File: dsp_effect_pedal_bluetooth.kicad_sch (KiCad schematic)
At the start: 1 part

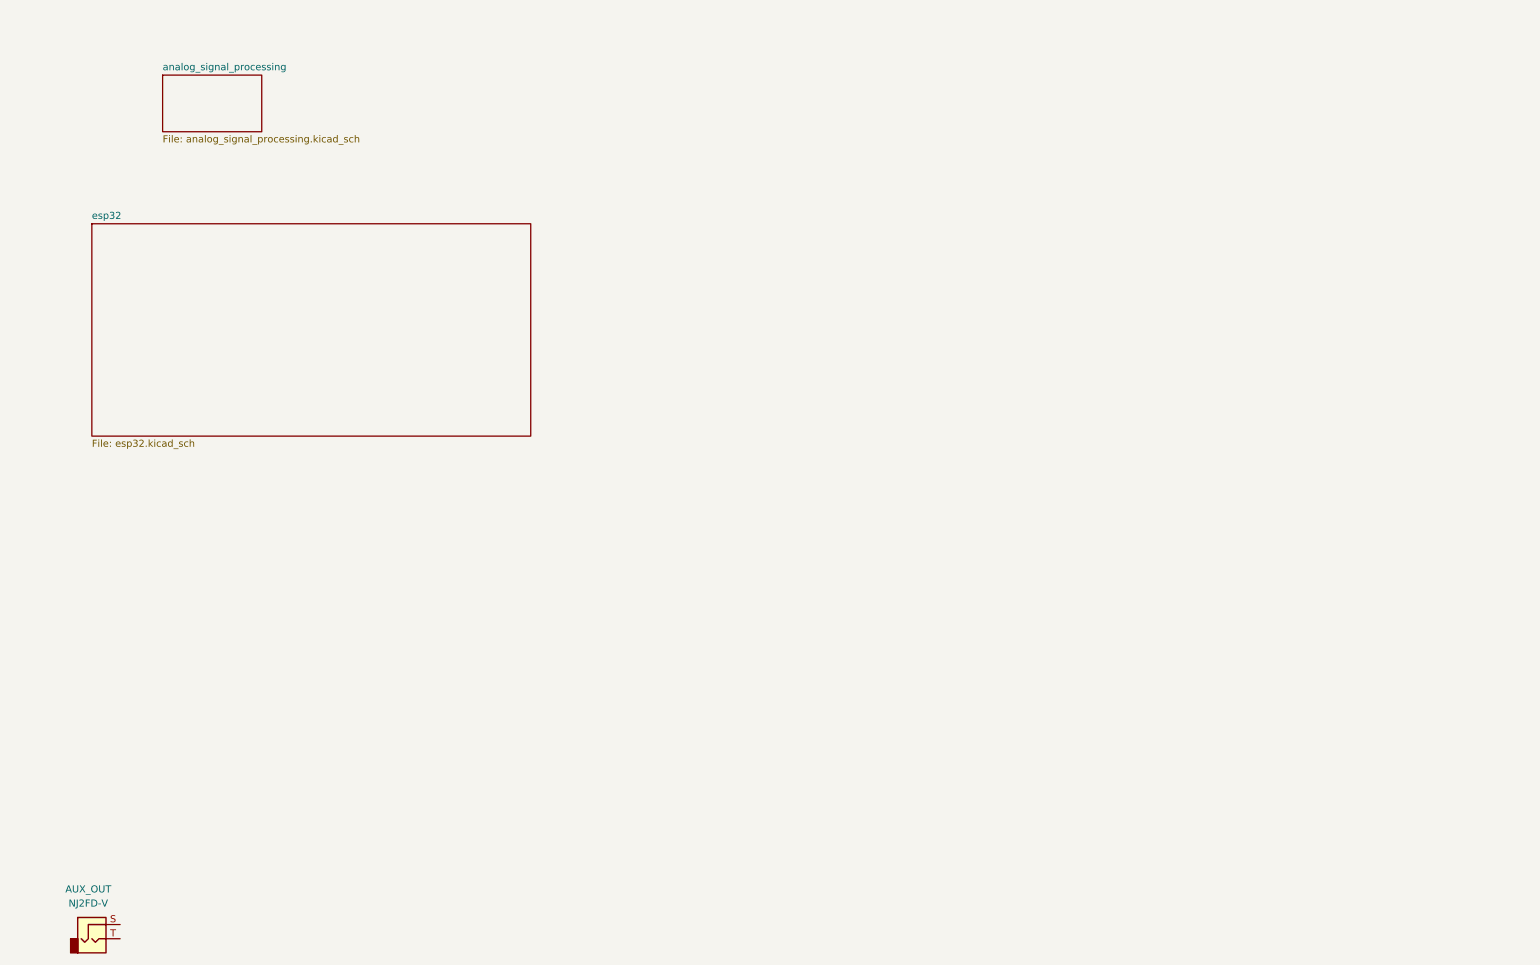
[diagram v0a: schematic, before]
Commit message: fixed a lot of things
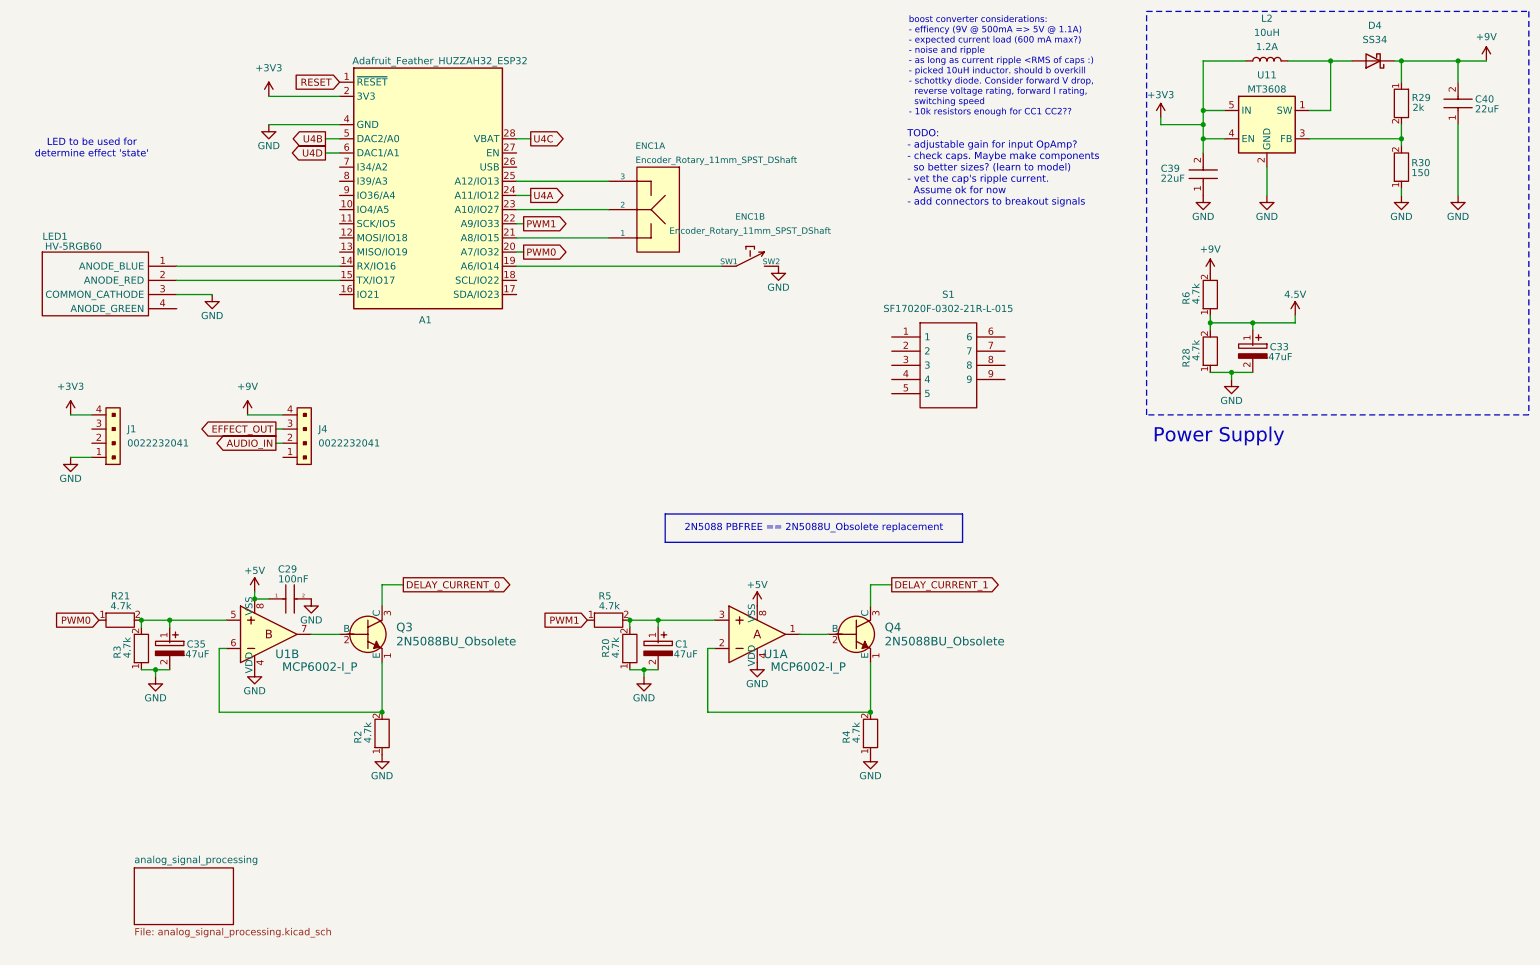
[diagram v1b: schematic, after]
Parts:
- removed AUX_OUT: NJ2FD-V, Connector_Audio:Jack_6.35mm_Neutrik_NJ2FD-V_Vertical, symbol Connector_Audio:NJ2FD-V
- added A1: Adafruit_Feather_HUZZAH32_ESP32, Module:Adafruit_Feather, symbol MCU_Module:Adafruit_Feather_HUZZAH32_ESP32
- added C1, C33, C35: 47uF, CAPPRD200W50D525H1250, symbol SamacSys_Parts:REA470M1CBK-0511P
- added C29: 100nF, SR211C104KARTR1, symbol SamacSys_Parts:SR211C104KARTR1
- added C39, C40: 22uF, FG20, symbol SamacSys_Parts:FG20X7R1C226MRT06
- added D4: SS34, Diode_SMD:D_SMA, symbol Diode:SS34
- added ENC1: Encoder_Rotary_11mm_SPST_DShaft, 4ms_Encoder:ENC_SPST_12mm, symbol PCM_4ms_Switch:Encoder_Rotary_11mm_SPST_DShaft
- added J1, J4: 0022232041, digikey-footprints:PinHeader_1x4_P2.54mm_Drill1.02mm, symbol dk_Rectangular-Connectors-Headers-Male-Pins:0022232041
- added L2: 10uH_1.0A_4018, Inductor_SMD:L_Taiyo-Yuden_NR-40xx, symbol PCM_4ms_Inductor:10uH_1.0A_4018
- added LED1: HV-5RGB60, HV5RGB25, symbol SamacSys_Parts:HV-5RGB60
- added Q3, Q4: 2N5088BU_Obsolete, digikey-footprints:TO-92-3, symbol dk_Transistors-Bipolar-BJT-Single:2N5088BU_Obsolete
- added R2, R20, R21, R28, R3, R4, R5, R6: 4.7k, RESAD1590W60L630D240, symbol SamacSys_Parts:MFR-25FRF52-4K7
- added R29: 2k, RESAD1550W60L630D230, symbol SamacSys_Parts:YR1B2K0CC
- added R30: 150, RESAD1590W60L630D240, symbol SamacSys_Parts:MFR-25FBF52-150R
- added S1: SF17020F-0302-21R-L-015, SF17020F030221RL015, symbol SamacSys_Parts:SF17020F-0302-21R-L-015
- added U1: MCP6002-I_P, digikey-footprints:DIP-8_W7.62mm, symbol dk_Linear-Amplifiers-Instrumentation-OP-Amps-Buffer-Amps:MCP6002-I_P
- added U11: MT3608, Package_TO_SOT_SMD:SOT-23-6, symbol Regulator_Switching:MT3608
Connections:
- new net: Q3.1 (E), R2.2, U1.6
- new net: Q4.1 (E), R4.2, U1.2
- new net: C35.1, R21.2, R3.2, U1.5
- new net: Q3.2 (B), U1.7
- new net: D4.2 (A), L2.2, U11.1 (SW)
- new net: Q4.2 (B), U1.1
- new net: A1.14 (RX/IO16), LED1.1 (ANODE_BLUE)
- new net: A1.15 (TX/IO17), LED1.2 (ANODE_RED)
- new net: C1.1, R20.2, R5.2, U1.3
- new net: A1.21 (A8/IO15), ENC1.1
- new net: A1.23 (A10/IO27), ENC1.2
- new net: A1.25 (A12/IO13), ENC1.3
- new net: R29.2, R30.2, U11.3 (FB)
- new net: A1.19 (A6/IO14), ENC1.SW1
- new net +3V3: A1.2 (3V3), C39.2, J1.4, L2.1, U11.4 (EN), U11.5 (IN)
- new net +5V: C29.1, U1.8 (VSS), U1.8 (VSS)
- new net +9V: C40.2, D4.1 (K), J4.4, R29.1, R6.2
- new net 4.5V: C33.1, R28.2, R6.1
- new net AUDIO_IN: J4.2
- new net DELAY_CURRENT_0: Q3.3 (C)
- new net DELAY_CURRENT_1: Q4.3 (C)
- new net EFFECT_OUT: J4.3
- new net GND: A1.4 (GND), C1.2, C29.2, C33.2, C35.2, C39.1, C40.1, ENC1.SW2, J1.1, LED1.3 (COMMON_CATHODE), R2.1, R20.1, R28.1, R3.1, R30.1, R4.1, U1.4 (VDD), U1.4 (VDD), U11.2 (GND)
- new net PWM0: A1.20 (A7/IO32), R21.1
- new net PWM1: A1.22 (A9/IO33), R5.1
- new net RESET: A1.1 (~{RESET})
- new net U4A: A1.24 (A11/IO12)
- new net U4B: A1.5 (DAC2/A0)
- new net U4C: A1.28 (VBAT)
- new net U4D: A1.6 (DAC1/A1)
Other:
- removed sheet esp32
- note added: "2N5088 PBFREE == 2N5088U_Obsolete replacement"
- note added: "LED to be used for determine effect 'state'"
- note added: "Power Supply"
- note added: "TODO: - adjustable gain for input OpAmp? - check caps. Maybe make components so better sizes? (learn to model) - vet the cap's ripple current. Assume ok for now - add connectors to breakout signals"
- note added: "boost converter considerations: - effiency (9V @ 500mA => 5V @ 1.1A) - expected current load (600 mA max?) - noise and ripple - as long as current ripple <RMS of caps :) - picked 10uH inductor. should b overkill - schottky diode. Consider forward V drop, reverse voltage rating, forward I rating, switching speed - 10k resistors enough for CC1 CC2??"
